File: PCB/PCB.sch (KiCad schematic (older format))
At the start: 2 parts

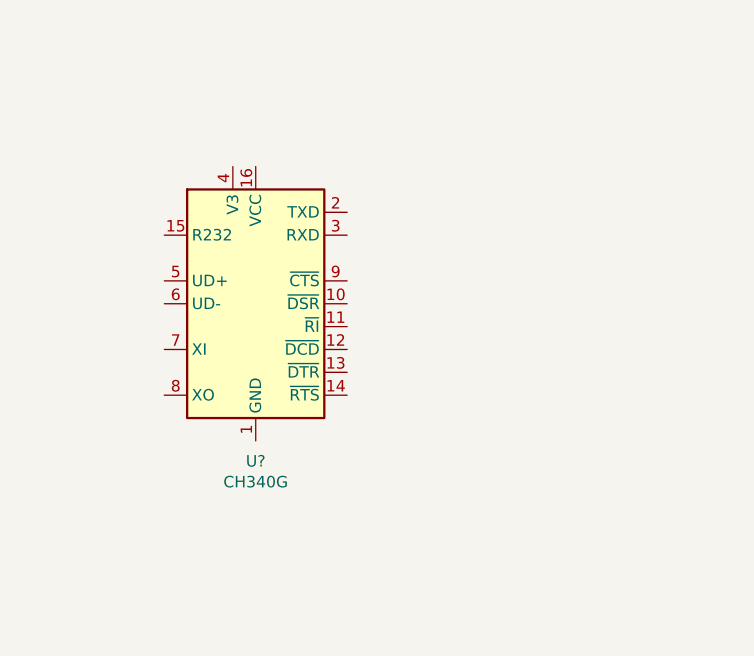
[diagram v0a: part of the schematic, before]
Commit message: footprint update
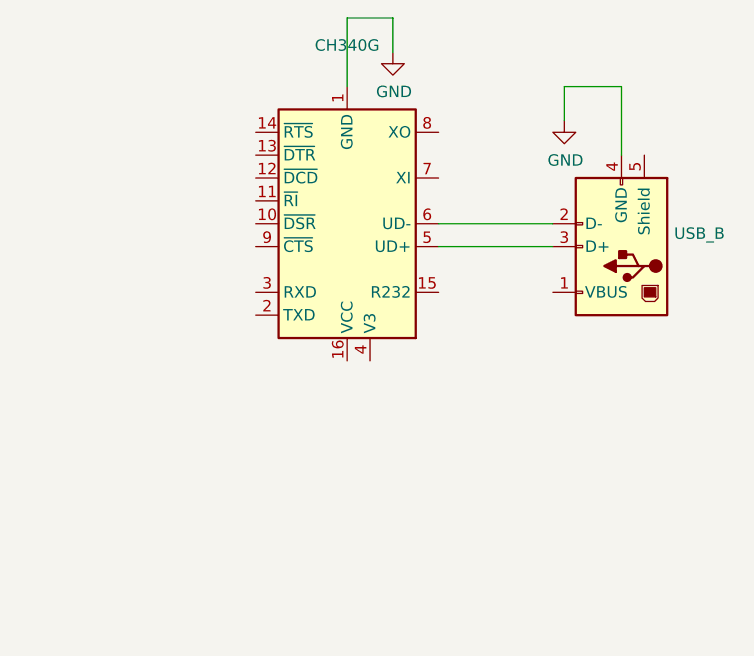
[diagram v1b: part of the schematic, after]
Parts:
- added J?: USB_B, Connector_USB:USB_B_OST_USB-B1HSxx_Horizontal, symbol Connector:USB_B
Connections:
- net GND: now reaches U?.1 (GND)
- net GND: now also J?.4 (GND)
- net at U?.5 (UD+): now also J?.3 (D+)
- net at U?.6 (UD-): now also J?.2 (D-)
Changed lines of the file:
@@
 EESchema Schematic File Version 4
+LIBS:PCB-cache
 EELAYER 30 0
 EELAYER END
@@
 L Interface_USB:CH340G U?
 U 1 1 5D6724AA
-P 8100 2150
-F 0 "U?" H 8100 1461 50  0000 C CNN
-F 1 "CH340G" H 8100 1370 50  0000 C CNN
-F 2 "Package_SO:SOIC-16_3.9x9.9mm_P1.27mm" H 8150 1600 50  0001 L CNN
-F 3 "http://www.datasheet5.com/pdf-local-2195953" H 7750 2950 50  0001 C CNN
-	1    8100 2150
+P 8500 1800
+F 0 "U?" H 8500 1111 50  0001 C CNN
+F 1 "CH340G" H 8500 1020 50  0000 C CNN
+F 2 "Package_SO:SOIC-16_3.9x9.9mm_P1.27mm" H 8550 1250 50  0001 L CNN
+F 3 "http://www.datasheet5.com/pdf-local-2195953" H 8150 2600 50  0001 C CNN
+	1    8500 1800
+	-1   0    0    1
+$EndComp
+$Comp
+L Connector:USB_B J?
+U 1 1 5D670289
+P 9700 1900
+F 0 "J?" H 9470 1797 50  0001 R CNN
+F 1 "USB_B" H 9470 1843 50  0000 R CNN
+F 2 "Connector_USB:USB_B_OST_USB-B1HSxx_Horizontal" H 9850 1850 50  0001 C CNN
+F 3 " ~" H 9850 1850 50  0001 C CNN
+	1    9700 1900
+	-1   0    0    1
+$EndComp
+$Comp
+L power:GND #PWR?
+U 1 1 5D677A17
+P 9450 1350
+F 0 "#PWR?" H 9450 1100 50  0001 C CNN
+F 1 "GND" H 9455 1177 50  0000 C CNN
+F 2 "" H 9450 1350 50  0001 C CNN
+F 3 "" H 9450 1350 50  0001 C CNN
+	1    9450 1350
 	1    0    0    -1
 $EndComp
+$Comp
+L power:GND #PWR?
+U 1 1 5D677FB5
+P 8700 1050
+F 0 "#PWR?" H 8700 800 50  0001 C CNN
+F 1 "GND" H 8705 877 50  0000 C CNN
+F 2 "" H 8700 1050 50  0001 C CNN
+F 3 "" H 8700 1050 50  0001 C CNN
+	1    8700 1050
+	1    0    0    -1
+$EndComp
+Wire Wire Line
+	9700 1500 9700 1200
+Wire Wire Line
+	9700 1200 9450 1200
+Wire Wire Line
+	9450 1200 9450 1350
+Wire Wire Line
+	8700 1050 8700 900
+Wire Wire Line
+	8700 900  8500 900
+Wire Wire Line
+	8500 900  8500 1200
+Wire Wire Line
+	8900 1800 9400 1800
+Wire Wire Line
+	9400 1900 8900 1900
 $EndSCHEMATC
